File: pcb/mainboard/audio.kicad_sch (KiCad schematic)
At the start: 41 parts, among them J701 AudioJack3_SwitchDualS, J702 AudioJack3_SwitchDualS, J703 DF13C-4P-1.25V, U701 WM8960, Y701 24.576MHz

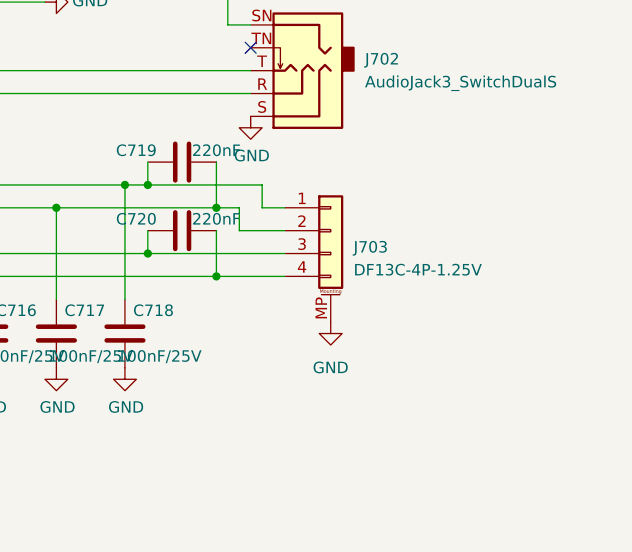
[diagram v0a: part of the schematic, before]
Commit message: pcb: r0.1 mb routing done
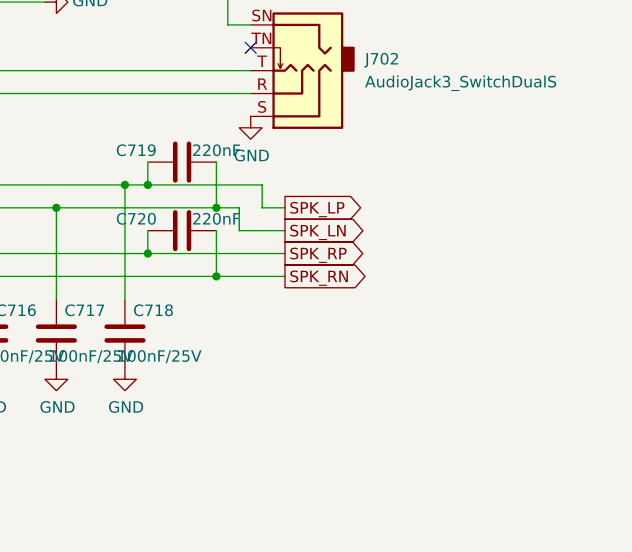
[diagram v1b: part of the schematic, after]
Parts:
- removed J703: DF13C-4P-1.25V, Connector_Hirose:Hirose_DF13C_CL535-0404-8-51_1x04-1MP_P1.25mm_Vertical, symbol Connector_Generic_MountingPin:Conn_01x04_MountingPin
- U701: footprint Package_DFN_QFN:QFN-32-1EP_5x5mm_P0.5mm_EP3.6x3.6mm_ThermalVias -> Package_DFN_QFN:QFN-32-1EP_5x5mm_P0.5mm_EP3.6x3.6mm
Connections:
- net SPK_LP: now reaches C718.2, C719.1, L703.2
- net SPK_LN: now reaches C717.2, C719.2, L704.2
- net SPK_RP: now reaches C716.2, C720.1, L705.2
- net SPK_RN: now reaches C714.2, C720.2, L706.2
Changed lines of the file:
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@@
+    )
+  )
+  (global_label "SPK_LP" (shape output) (at 210.82 119.38 0) (fields_autoplaced)
+    (effects (font (size 1.27 1.27)) (justify left))
+    (property "Intersheet References" "${INTERSHEET_REFS}" (id 0) (at 220.2483 119.3006 0)
+      (effects (font (size 1.27 1.27)) (justify left) hide)
+    )
+  )
+  (global_label "SPK_LN" (shape output) (at 210.82 121.92 0) (fields_autoplaced)
+    (effects (font (size 1.27 1.27)) (justify left))
+    (property "Intersheet References" "${INTERSHEET_REFS}" (id 0) (at 220.3088 121.8406 0)
+      (effects (font (size 1.27 1.27)) (justify left) hide)
+    )
+  )
+  (global_label "SPK_RP" (shape output) (at 210.82 124.46 0) (fields_autoplaced)
+    (effects (font (size 1.27 1.27)) (justify left))
+    (property "Intersheet References" "${INTERSHEET_REFS}" (id 0) (at 220.4902 124.3806 0)
+      (effects (font (size 1.27 1.27)) (justify left) hide)
+    )
+  )
+  (global_label "SPK_RN" (shape output) (at 210.82 127 0) (fields_autoplaced)
+    (effects (font (size 1.27 1.27)) (justify left))
+    (property "Intersheet References" "${INTERSHEET_REFS}" (id 0) (at 220.5507 126.9206 0)
+      (effects (font (size 1.27 1.27)) (justify left) hide)
     )
   )
@@
     )
     (property "Datasheet" "" (id 3) (at 207.01 109.22 0)
-      (effects (font (size 1.27 1.27)) hide)
-    )
-    (pin "1")
-  )
-  (symbol (lib_id "power:GND") (at 215.9 132.08 0) (unit 1)
-    (in_bom yes) (on_board yes) (fields_autoplaced)
-    (property "Reference" "#PWR0113" (id 0) (at 215.9 138.43 0)
-      (effects (font (size 1.27 1.27)) hide)
-    )
-    (property "Value" "GND" (id 1) (at 215.9 137.16 0))
-    (property "Footprint" "" (id 2) (at 215.9 132.08 0)
-      (effects (font (size 1.27 1.27)) hide)
-    )
-    (property "Datasheet" "" (id 3) (at 215.9 132.08 0)
       (effects (font (size 1.27 1.27)) hide)
     )
@@
     (pin "1")
     (pin "2")
-  )
-  (symbol (lib_id "Connector_Generic_MountingPin:Conn_01x04_MountingPin") (at 215.9 121.92 0) (unit 1)
-    (in_bom yes) (on_board yes) (fields_autoplaced)
-    (property "Reference" "J703" (id 0) (at 218.44 123.7614 0)
-      (effects (font (size 1.27 1.27)) (justify left))
-    )
-    (property "Value" "DF13C-4P-1.25V" (id 1) (at 218.44 126.3014 0)
-      (effects (font (size 1.27 1.27)) (justify left))
-    )
-    (property "Footprint" "Connector_Hirose:Hirose_DF13C_CL535-0404-8-51_1x04-1MP_P1.25mm_Vertical" (id 2) (at 215.9 121.92 0)
-      (effects (font (size 1.27 1.27)) hide)
-    )
-    (property "Datasheet" "~" (id 3) (at 215.9 121.92 0)
-      (effects (font (size 1.27 1.27)) hide)
-    )
-    (property "LCSC" "C116890" (id 4) (at 215.9 121.92 0)
-      (effects (font (size 1.27 1.27)) hide)
-    )
-    (property "Ref.Price" "0.1932" (id 5) (at 215.9 121.92 0)
-      (effects (font (size 1.27 1.27)) hide)
-    )
-    (pin "1")
-    (pin "2")
-    (pin "3")
-    (pin "4")
-    (pin "MP")
   )
   (symbol (lib_id "symbols:AudioJack3_SwitchDualS") (at 82.55 121.92 0) (mirror x) (unit 1)
@@
     (property "Reference" "U701" (id 0) (at 142.24 72.009 0))
     (property "Value" "WM8960" (id 1) (at 142.24 74.3204 0))
-    (property "Footprint" "Package_DFN_QFN:QFN-32-1EP_5x5mm_P0.5mm_EP3.6x3.6mm_ThermalVias" (id 2) (at 142.24 73.66 0)
-      (effects (font (size 1.27 1.27)) hide)
-    )
+    (property "Footprint" "Package_DFN_QFN:QFN-32-1EP_5x5mm_P0.5mm_EP3.6x3.6mm" (id 2) (at 142.24 73.66 0)
+      (effects (font (size 1.27 1.27)) hide)
+    )
